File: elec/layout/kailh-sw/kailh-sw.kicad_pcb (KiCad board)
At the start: 2 copper layers, 40 x 40 mm, 0 parts

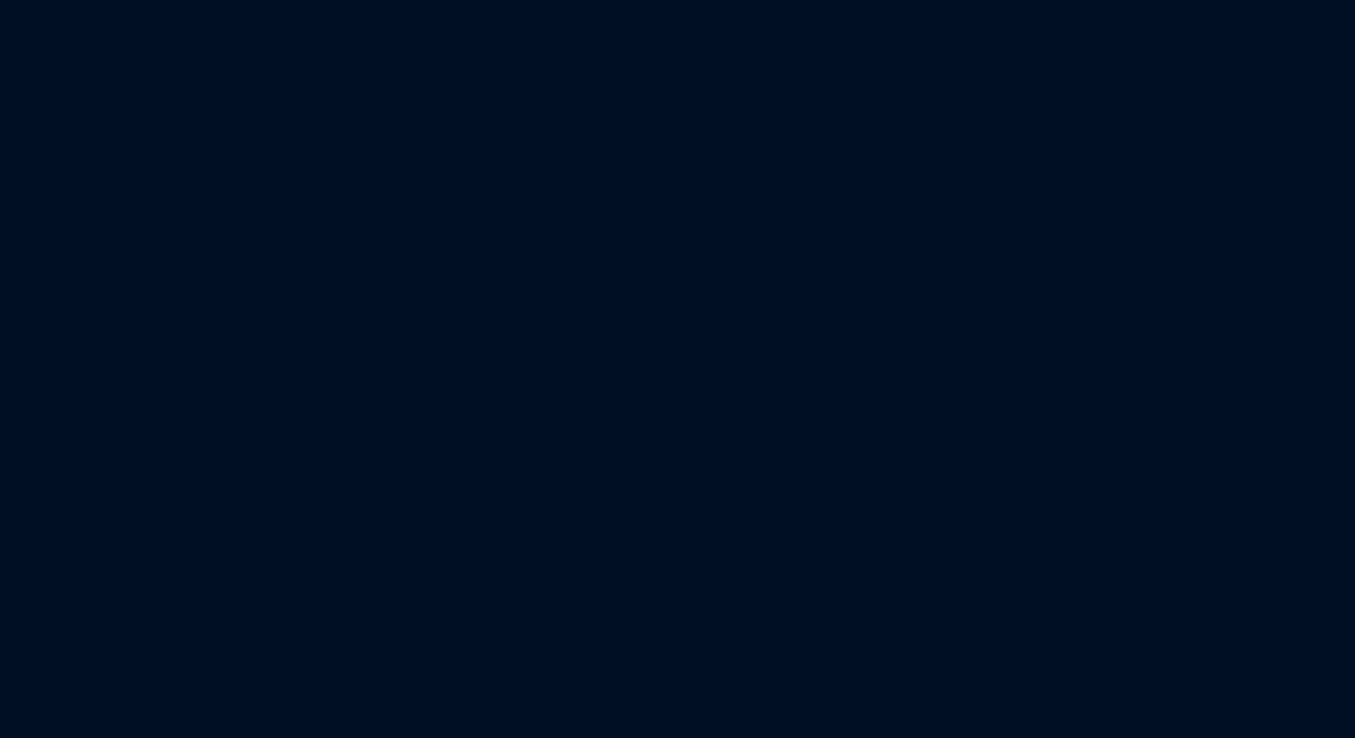
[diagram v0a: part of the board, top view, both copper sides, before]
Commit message: :woozy:
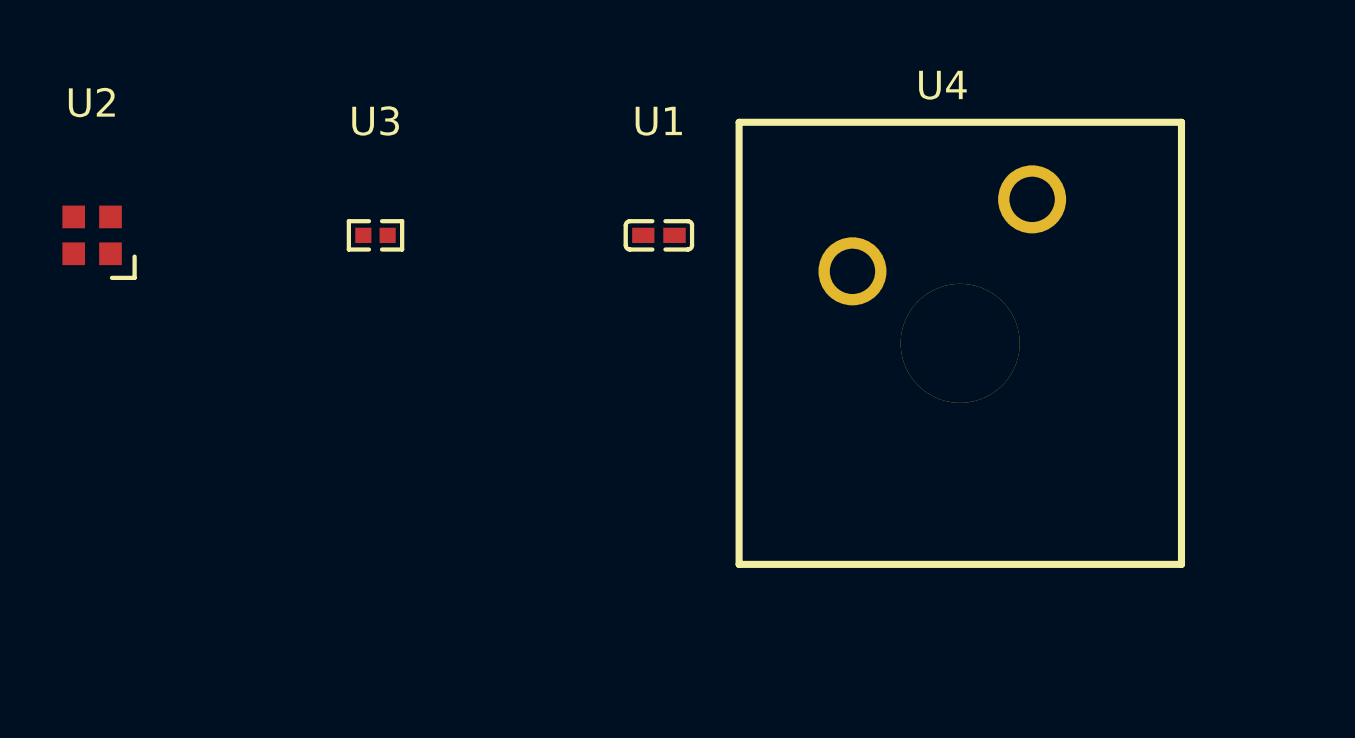
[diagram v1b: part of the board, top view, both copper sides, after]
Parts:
- added U1: 100nF ±10% 16V X7R, atopile:C0402-b3ef17, F.Cu at (30.0, -5.00)
- added U2: , lib:LED-SMD_4P-L2.0-W2.0-BR, F.Cu at (10.0, -5.00)
- added U3: 10kΩ ±1% 62.5mW, atopile:R0402-56259e, F.Cu at (20.0, -5.00)
- added U4: , lib:KEY-TH_CPG1511F01S0X, F.Cu at (40.0, -5.00)
